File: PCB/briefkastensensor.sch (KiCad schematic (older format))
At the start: 19 parts, among them J1 Conn_01x02, J2 AVR-ISP-6, SW1 SW_DIP_x02, SW2 Reset, U1 ATtiny84-20PU, U2 RFM95W

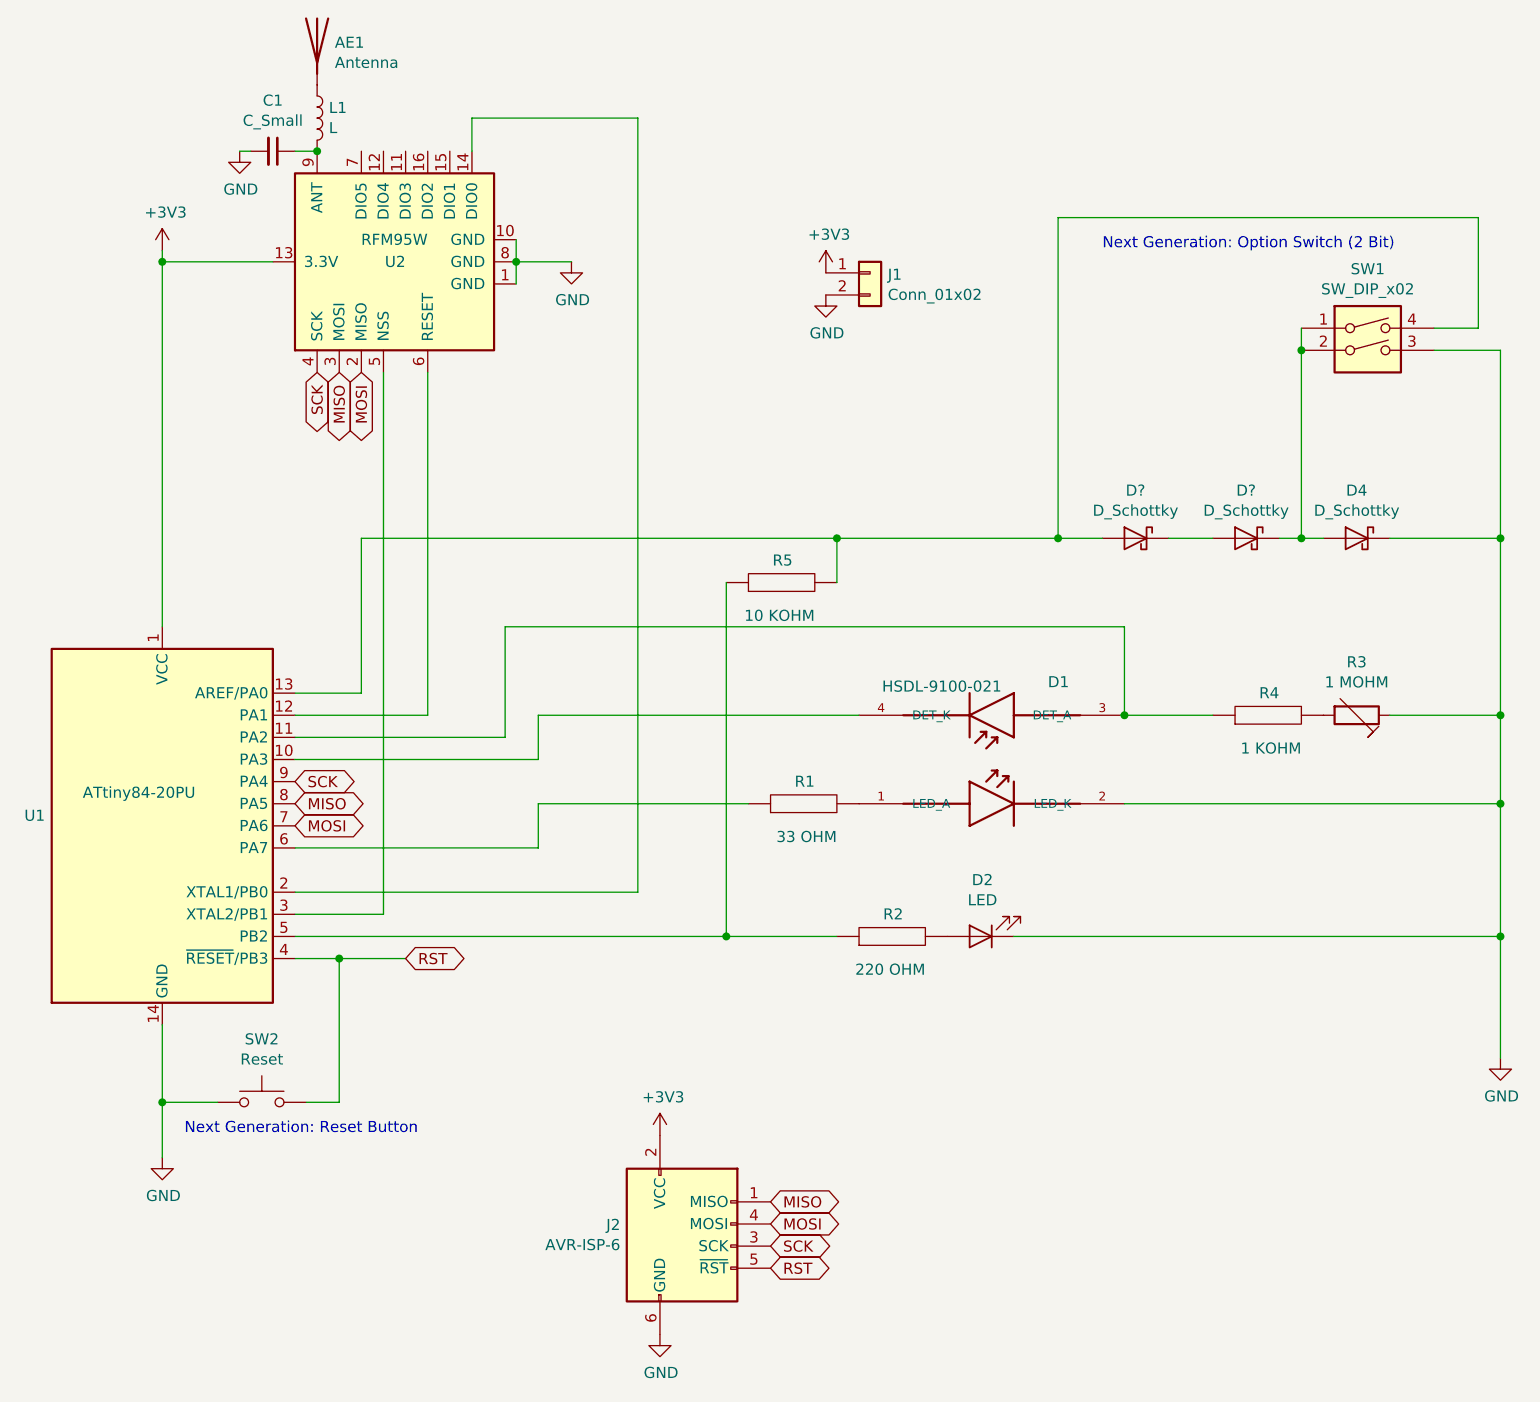
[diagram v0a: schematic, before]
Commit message: whitespace fixes
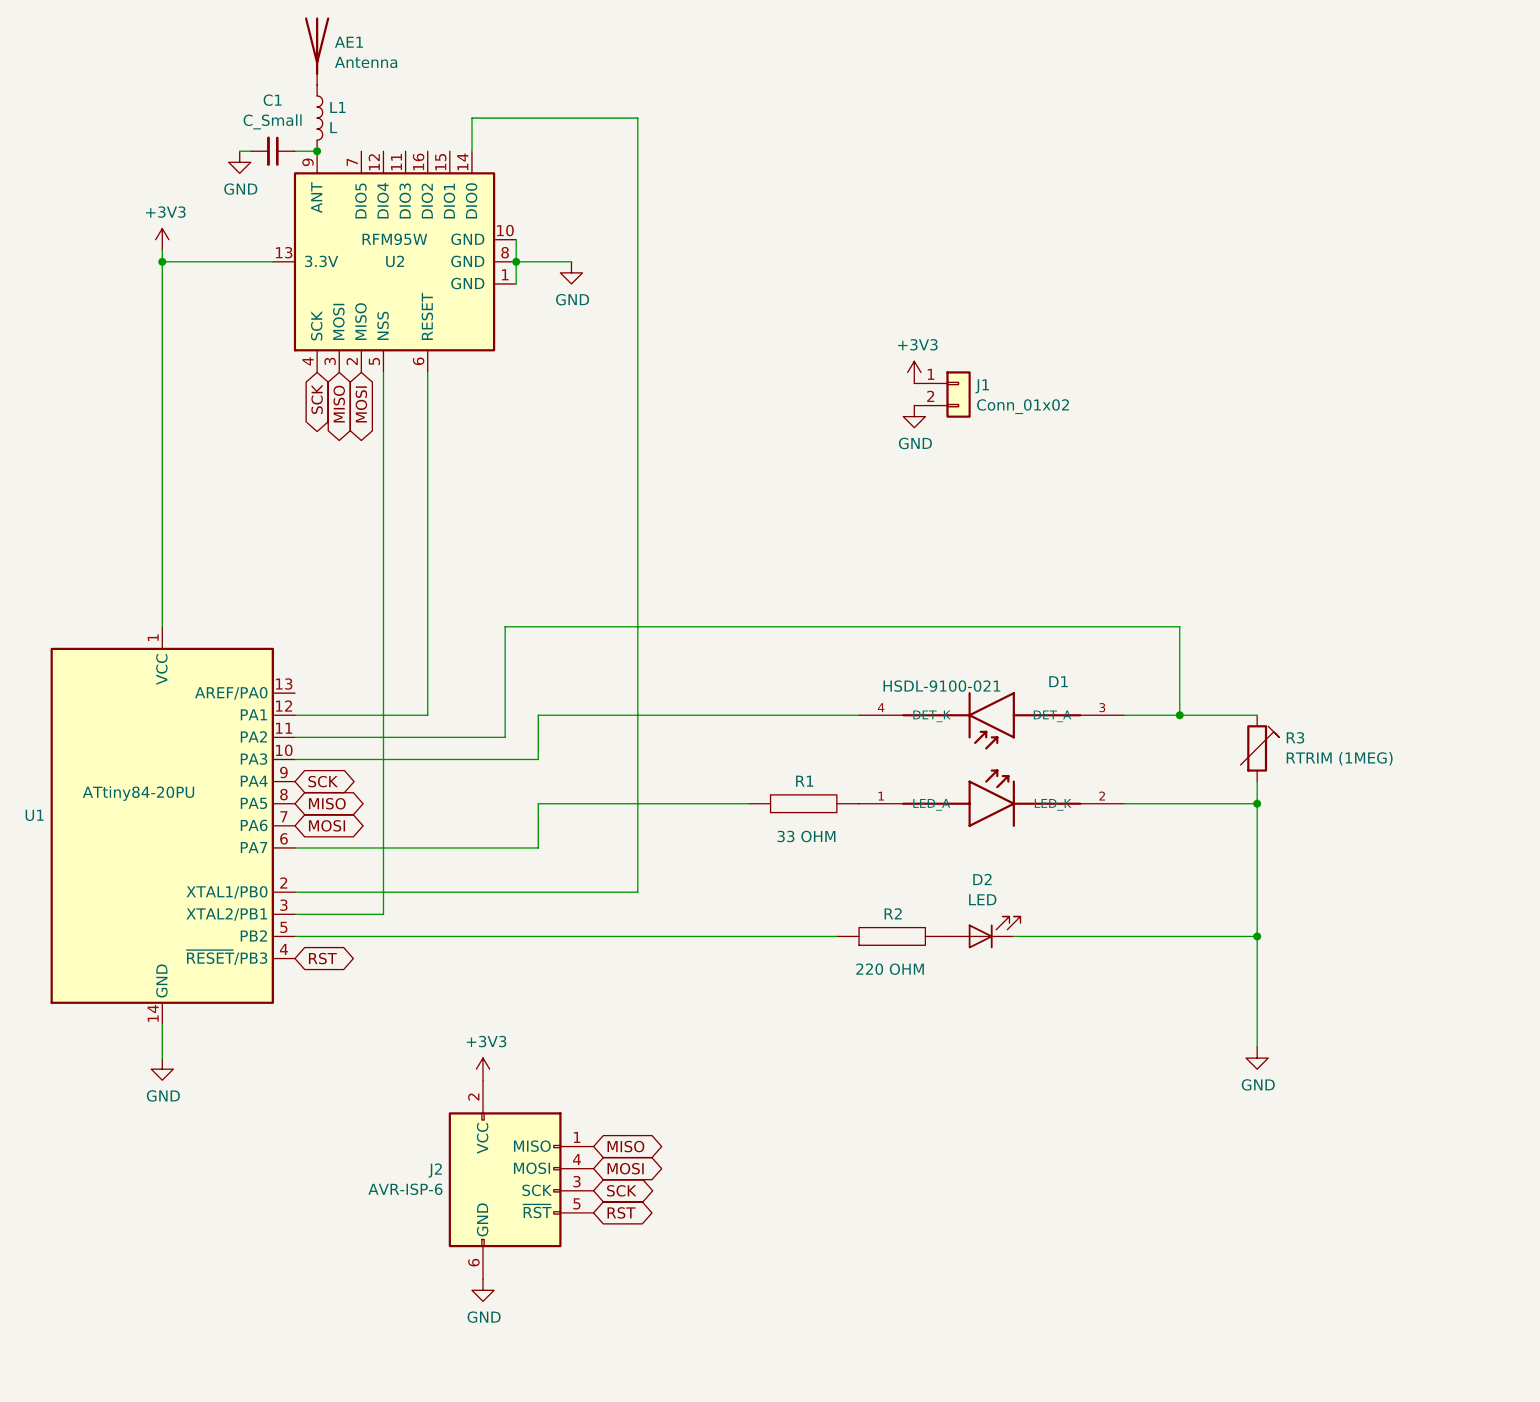
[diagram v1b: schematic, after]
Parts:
- removed D4, D? (x2): D_Schottky, symbol Device:D_Schottky
- removed R4: 1 KOHM, Resistor_SMD:R_1206_3216Metric, symbol pspice:R
- removed R5: 10 KOHM, Resistor_SMD:R_1206_3216Metric, symbol pspice:R
- removed SW1: SW_DIP_x02, symbol Switch:SW_DIP_x02
- removed SW2: Reset, symbol Switch:SW_Push
- R3: value 1 MOHM -> RTRIM (1MEG); footprint (none) -> Potentiometer_SMD:Potentiometer_Bourns_3314G_Vertical
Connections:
- net GND: now also R3.2; no longer R3.1
- net at D1.3 (DET_A), U1.11 (PA2): now also R3.1
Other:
- note removed: "Next Generation: Option Switch (2 Bit)"
- note removed: "Next Generation: Reset Button"
- moved on the sheet: J1, J2
